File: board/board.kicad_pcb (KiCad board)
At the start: 2 copper layers, 21 x 13 mm, 1 part

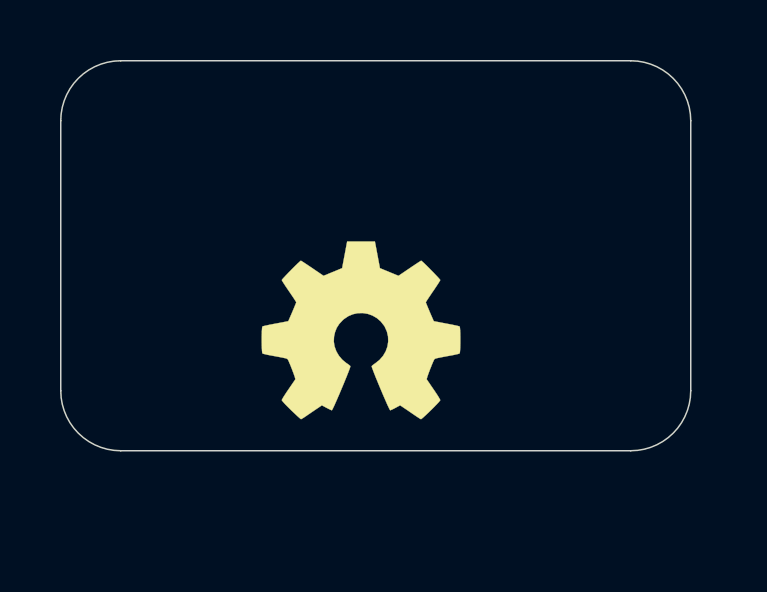
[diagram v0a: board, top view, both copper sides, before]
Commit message: initial
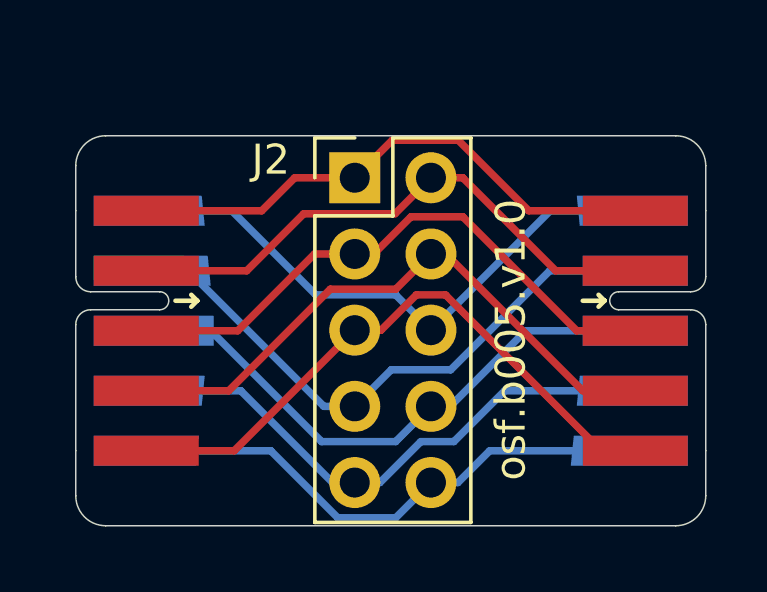
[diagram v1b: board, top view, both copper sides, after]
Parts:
- removed LOGO1: Logo_Open_Hardware_Small, Symbol:OSHW-Symbol_6.7x6mm_SilkScreen
- added J1: Conn_01x10_Male, on_edge:on_edge_2x05_device, F.Cu at (140.5, 99.0)
- added J2: CA2310PA10Z, Connector_PinHeader_2.54mm:PinHeader_2x05_P2.54mm_Vertical, F.Cu at (149.8, 93.9)
- added J6: Conn_01x10_Male, on_edge:on_edge_2x05_host, F.Cu at (161.5, 99.0)
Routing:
- net Net-(J1-Pad5): track 0.00 -> 20.6 mm
- net Net-(J1-Pad7): track 0.00 -> 20.3 mm
- net Net-(J1-Pad4): track 0.00 -> 20.1 mm
- net Net-(J1-Pad6): track 0.00 -> 19.5 mm
- net Net-(J1-Pad3): track 0.00 -> 19.4 mm
- net Net-(J1-Pad8): track 0.00 -> 19.1 mm
- net Net-(J1-Pad2): track 0.00 -> 18.9 mm
- net Net-(J1-Pad9): track 0.00 -> 18.7 mm
- net Net-(J1-Pad1): track 0.00 -> 18.2 mm
- net Net-(J1-Pad10): track 0.00 -> 18.1 mm
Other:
- outline, holes or cut-outs redrawn
- copper layers 2 -> 4
- rule pad_to_mask_clearance: 0 -> 0.051
- board text added: "osf.b005.v1.0"
